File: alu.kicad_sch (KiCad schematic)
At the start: 41 parts, among them J0 640-USB4970-00-A, SW0 SW_DIP_x04, SW1 SW_DIP_x04, SW2 SW_DIP_x04, U0 SN74LS08N, U1 SN74HC86N, U2 SN74HC86N, U3 SN74LS08N, U4 SN74LS08N, U5 CD74HCT32E

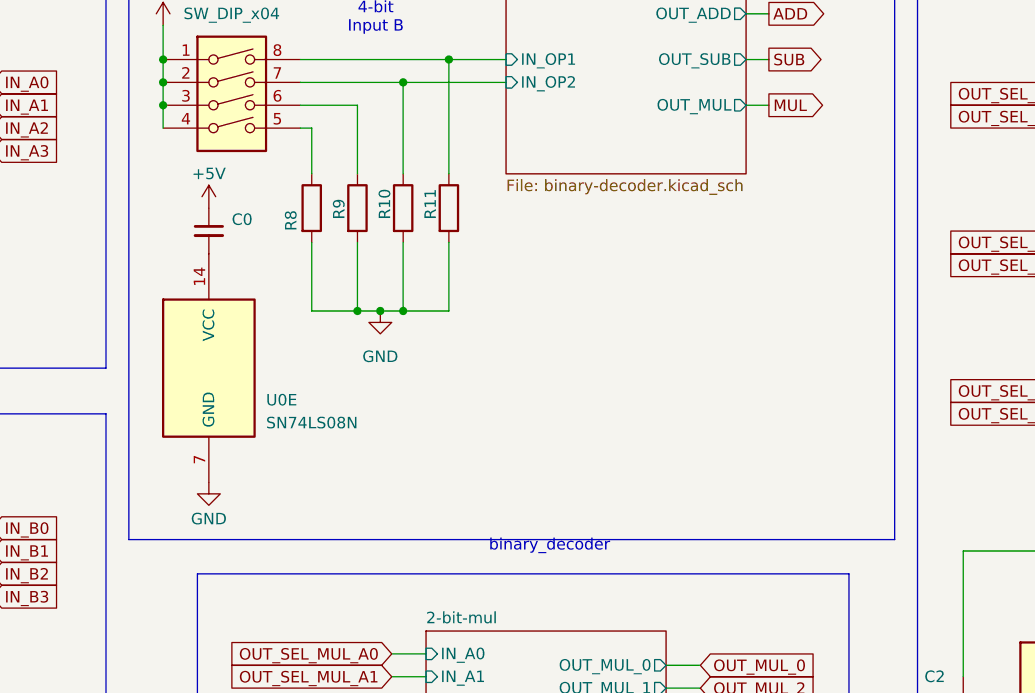
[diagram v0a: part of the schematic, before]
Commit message: fix: 0 error 0 warning
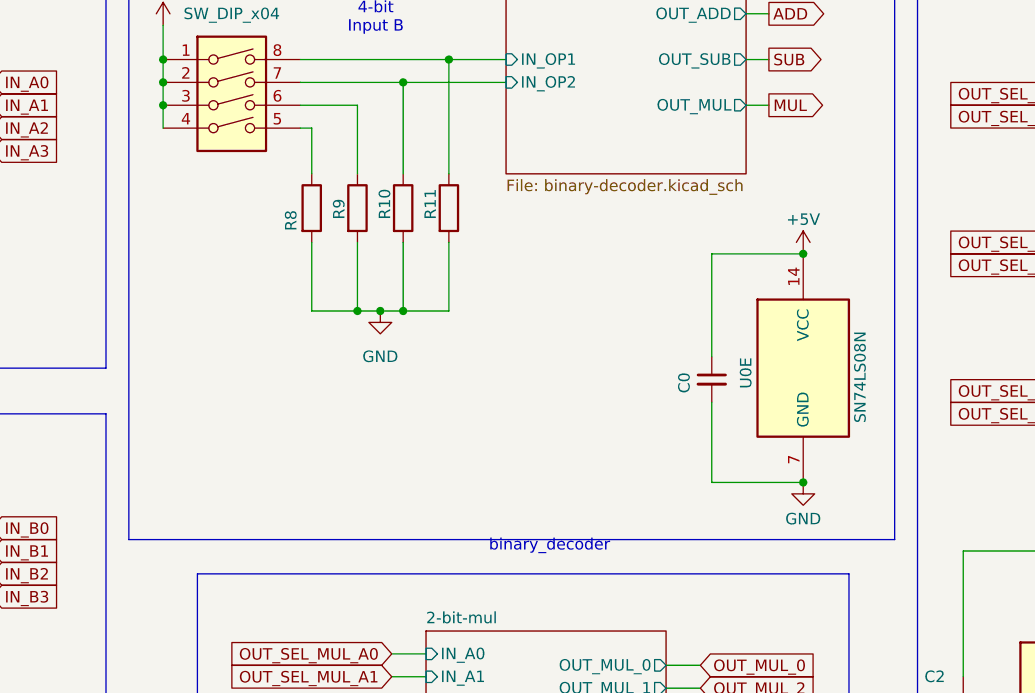
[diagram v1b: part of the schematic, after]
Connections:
- net +5V: now also U0.14 (VCC)
- net GND: now also C0.2
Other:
- moved on the sheet: C0, U0E
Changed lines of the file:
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@@
 	)
 	(junction
+		(at 149.86 74.93)
+		(diameter 0)
+		(color 0 0 0 0)
+	)
+	(junction
 		(at 105.41 30.48)
 		(diameter 0)
@@
 	)
 	(junction
+		(at 149.86 49.53)
+		(diameter 0)
+		(color 0 0 0 0)
+	)
+	(junction
 		(at 267.97 137.16)
 		(diameter 0)
@@
 	(wire
 		(pts
+			(xy 139.7 66.04) (xy 139.7 74.93)
+		)
+		(stroke
+			(width 0)
+			(type default)
+		)
+	)
+	(wire
+		(pts
 			(xy 41.91 46.99) (xy 41.91 54.61)
 		)
@@
 	(wire
 		(pts
+			(xy 149.86 49.53) (xy 139.7 49.53)
+		)
+		(stroke
+			(width 0)
+			(type default)
+		)
+	)
+	(wire
+		(pts
 			(xy 184.15 16.51) (xy 186.69 16.51)
 		)
@@
 	(wire
 		(pts
+			(xy 139.7 49.53) (xy 139.7 60.96)
+		)
+		(stroke
+			(width 0)
+			(type default)
+		)
+	)
+	(wire
+		(pts
 			(xy 231.14 82.55) (xy 231.14 97.79)
 		)
@@
 	(wire
 		(pts
+			(xy 139.7 74.93) (xy 149.86 74.93)
+		)
+		(stroke
+			(width 0)
+			(type default)
+		)
+	)
+	(wire
+		(pts
 			(xy 46.99 88.9) (xy 46.99 82.55)
 		)
@@
 	(symbol
 		(lib_id "power:GND")
-		(at 83.82 74.93 0)
+		(at 149.86 74.93 0)
 		(unit 1)
 		(body_style 1)
@@
 		(dnp no)
 		(property "Reference" "#PWR06"
-			(at 83.82 81.28 0)
+			(at 149.86 81.28 0)
 			(hide yes)
 			(show_name no)
@@
 		)
 		(property "Value" "GND"
-			(at 83.82 78.994 0)
+			(at 149.86 78.994 0)
 			(show_name no)
 			(do_not_autoplace no)
@@
 		)
 		(property "Footprint" ""
-			(at 83.82 74.93 0)
+			(at 149.86 74.93 0)
 			(hide yes)
 			(show_name no)
@@
 		)
 		(property "Datasheet" ""
-			(at 83.82 74.93 0)
+			(at 149.86 74.93 0)
 			(hide yes)
 			(show_name no)
@@
 		)
 		(property "Description" "Power symbol creates a global label with name \"GND\" , ground"
-			(at 83.82 74.93 0)
+			(at 149.86 74.93 0)
 			(hide yes)
 			(show_name no)
@@
 	(symbol
 		(lib_id "74xx:74LS08")
-		(at 83.82 62.23 0)
+		(at 149.86 62.23 0)
 		(unit 5)
 		(body_style 1)
@@
 		(dnp no)
 		(property "Reference" "U0"
-			(at 90.17 65.786 0)
+			(at 143.51 64.516 90)
 			(show_name no)
 			(do_not_autoplace no)
@@
 		)
 		(property "Value" "SN74LS08N"
-			(at 90.17 68.326 0)
+			(at 156.21 68.326 90)
 			(show_name no)
 			(do_not_autoplace no)
@@
 		)
 		(property "Footprint" "Package_DIP:DIP-14_W7.62mm_LongPads"
-			(at 83.82 62.23 0)
+			(at 149.86 62.23 0)
 			(hide yes)
 			(show_name no)
@@
 		)
 		(property "Datasheet" "https://www.ti.com/lit/ds/symlink/sn74hc86.pdf"
-			(at 83.82 62.23 0)
+			(at 149.86 62.23 0)
 			(hide yes)
 			(show_name no)
@@
 		)
 		(property "Description" "Quad And2"
-			(at 83.82 62.23 0)
+			(at 149.86 62.23 0)
 			(hide yes)
 			(show_name no)
@@
 	(symbol
 		(lib_id "power:+5V")
-		(at 83.82 44.45 0)
+		(at 149.86 49.53 0)
 		(unit 1)
 		(body_style 1)
@@
 		(dnp no)
 		(property "Reference" "#PWR05"
-			(at 83.82 48.26 0)
+			(at 149.86 53.34 0)
 			(hide yes)
 			(show_name no)
@@
 		)
 		(property "Value" "+5V"
-			(at 83.82 40.64 0)
+			(at 149.86 45.72 0)
 			(show_name no)
 			(do_not_autoplace no)
@@
 		)
 		(property "Footprint" ""
-			(at 83.82 44.45 0)
+			(at 149.86 49.53 0)
 			(hide yes)
 			(show_name no)
@@
 		)
 		(property "Datasheet" ""
-			(at 83.82 44.45 0)
+			(at 149.86 49.53 0)
 			(hide yes)
 			(show_name no)
@@
 		)
 		(property "Description" "Power symbol creates a global label with name \"+5V\""
-			(at 83.82 44.45 0)
+			(at 149.86 49.53 0)
 			(hide yes)
 			(show_name no)
@@
 	(symbol
 		(lib_id "Device:C_Small")
-		(at 83.82 46.99 0)
+		(at 139.7 63.5 0)
 		(unit 1)
 		(body_style 1)
@@
 		(in_pos_files yes)
 		(dnp no)
-		(fields_autoplaced yes)
 		(property "Reference" "C0"
-			(at 86.36 45.7262 0)
+			(at 136.652 65.024 90)
 			(show_name no)
 			(do_not_autoplace no)
@@
 		)
 		(property "Value" "CC0603KRX7R9BB104"
-			(at 86.36 48.2662 0)
+			(at 142.24 64.7762 0)
 			(hide yes)
 			(show_name no)
@@
 		)
 		(property "Footprint" "Capacitor_SMD:C_0603_1608Metric_Pad1.08x0.95mm_HandSolder"
-			(at 83.82 46.99 0)
+			(at 139.7 63.5 0)
 			(hide yes)
 			(show_name no)
@@
 		)
 		(property "Datasheet" ""
-			(at 83.82 46.99 0)
+			(at 139.7 63.5 0)
 			(hide yes)
 			(show_name no)
@@
 		)
 		(property "Description" "Unpolarized capacitor, small symbol"
-			(at 83.82 46.99 0)
+			(at 139.7 63.5 0)
 			(hide yes)
 			(show_name no)
